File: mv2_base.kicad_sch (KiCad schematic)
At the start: 60 parts, among them J1 Conn_01x20, J2 OLED, U1 TPS65130RGE

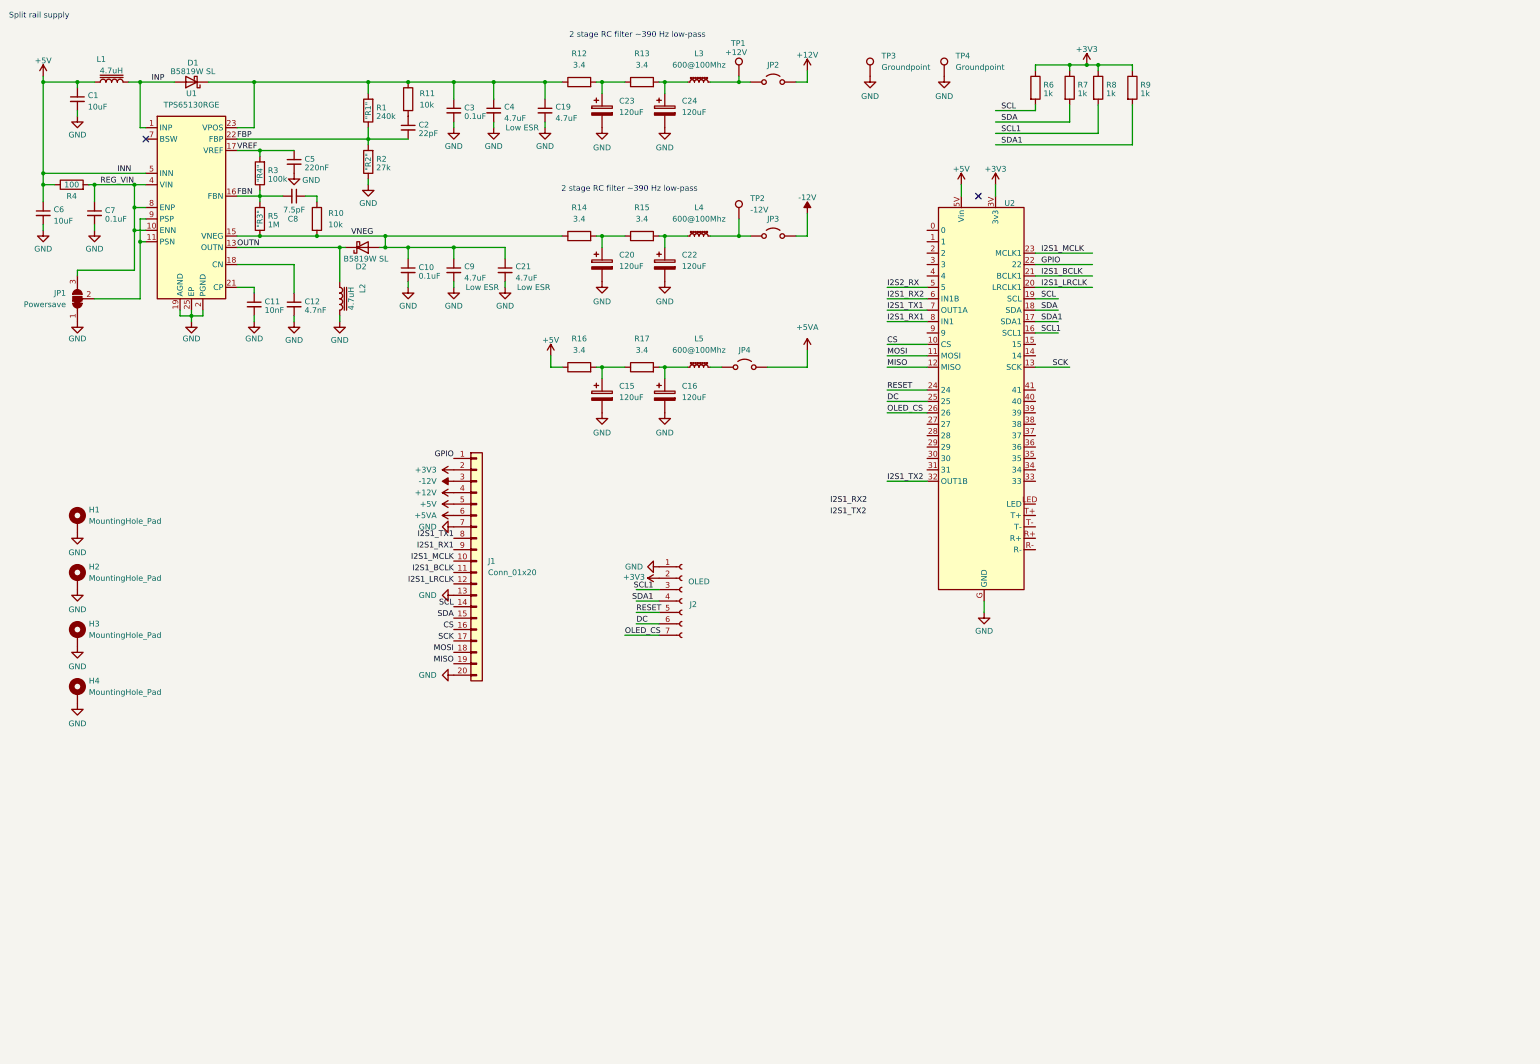
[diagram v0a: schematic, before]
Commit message: New filters
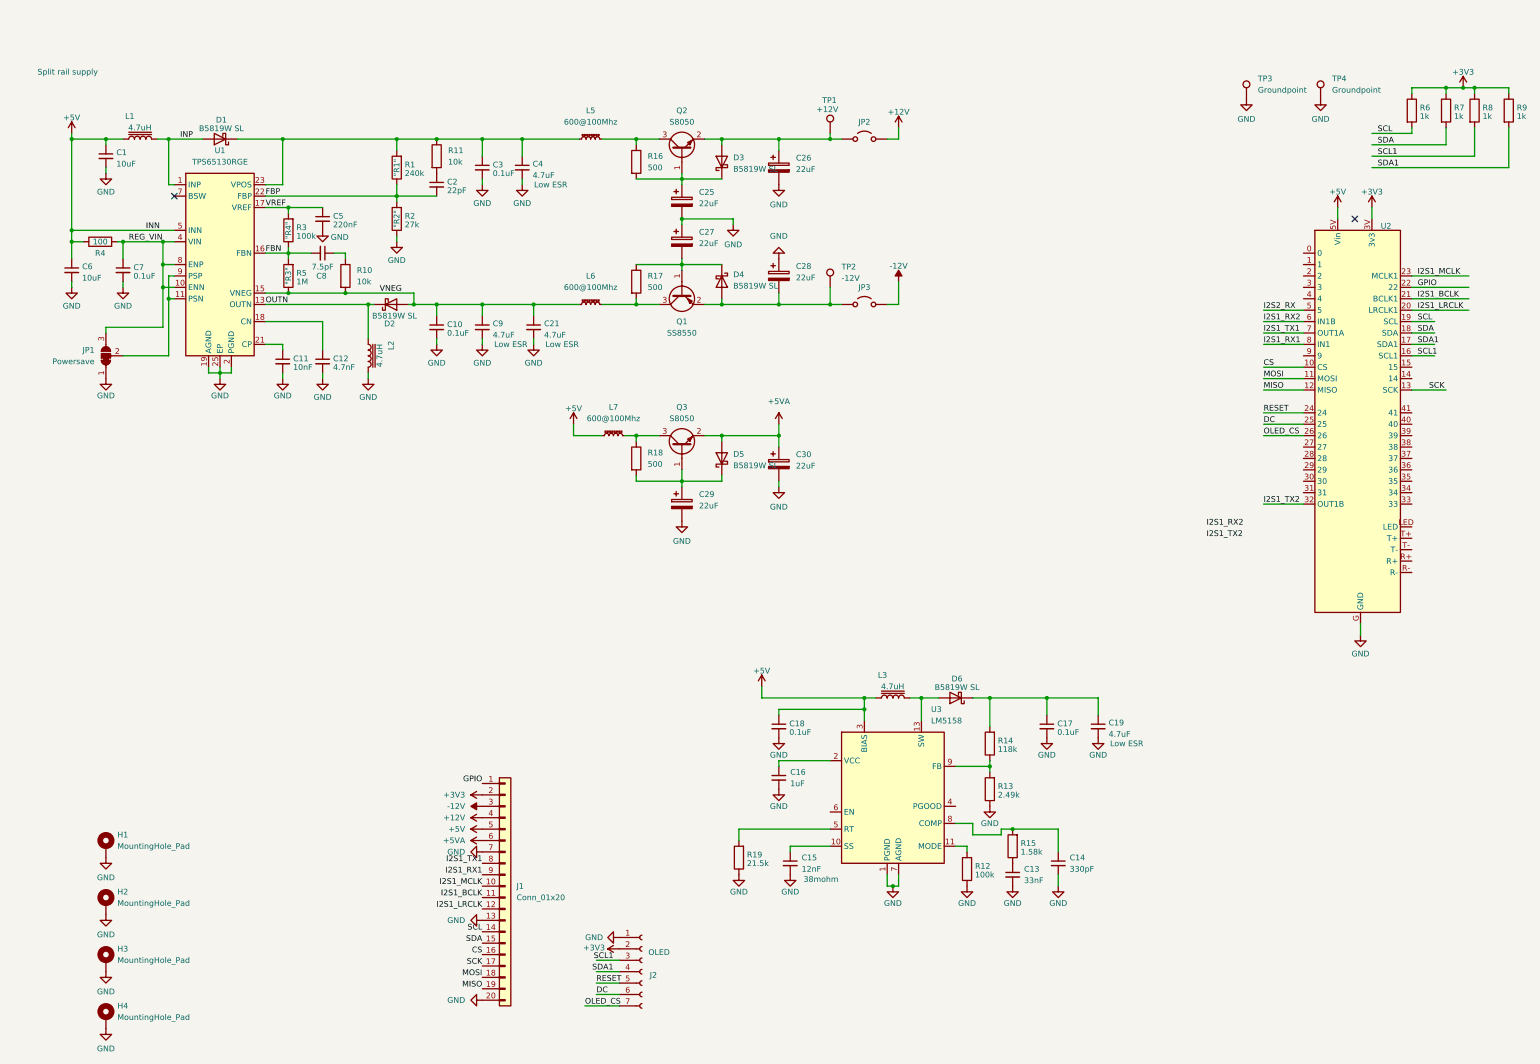
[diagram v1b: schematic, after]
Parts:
- removed C15, C16, C20, C22, C23, C24: 120uF, Capacitor_SMD:CP_Elec_6.3x7.7, symbol Device:C_Polarized
- removed JP4: Jumper_2_Open, Connector_PinHeader_2.54mm:PinHeader_1x02_P2.54mm_Vertical, symbol Jumper:Jumper_2_Open
- removed L3, L4: 600@100Mhz, Inductor_SMD:L_0603_1608Metric, symbol Device:L_Ferrite_Small
- added C13: 33nF, Capacitor_SMD:C_0603_1608Metric_Pad1.08x0.95mm_HandSolder, symbol Device:C_Small
- added C14: 330pF, Capacitor_SMD:C_0603_1608Metric_Pad1.08x0.95mm_HandSolder, symbol Device:C_Small
- added C15: 12nF, Capacitor_SMD:C_0603_1608Metric_Pad1.08x0.95mm_HandSolder, symbol Device:C_Small
- added C16: 1uF, Capacitor_SMD:C_0805_2012Metric_Pad1.18x1.45mm_HandSolder, symbol Device:C_Small
- added C17, C18: 0.1uF, Capacitor_SMD:C_0402_1005Metric, symbol Device:C_Small
- added C25, C26, C27, C28, C29, C30: 22uF, Capacitor_SMD:C_0805_2012Metric, symbol Device:C_Polarized
- added D3, D4, D5, D6: B5819W SL, Diode_SMD:D_SOD-123, symbol Device:D_Schottky
- added L3: 4.7uH, Inductor_SMD:L_Wuerth_WE-TPC-3816, symbol Device:L_Iron
- added L6, L7: 600@100Mhz, Inductor_SMD:L_0603_1608Metric, symbol Device:L_Ferrite_Small
- added Q1: SS8550, Package_TO_SOT_SMD:SOT-23, symbol Transistor_BJT:Q_PNP_BEC
- added Q2, Q3: S8050, Package_TO_SOT_SMD:SOT-23, symbol Transistor_BJT:Q_NPN_BEC
- added R18: 500, Resistor_SMD:R_0402_1005Metric, symbol Device:R
- added R19: 21.5k, Resistor_SMD:R_0402_1005Metric, symbol Device:R
- added U3: LM5158, symbol Library:LM5158
- C19: footprint Capacitor_SMD:C_0805_2012Metric_Pad1.18x1.45mm_HandSolder -> Capacitor_SMD:C_0805_2012Metric; DatasheetRef C4 -> C5
- R12: value 3.4 -> 100k; footprint Resistor_SMD:R_0603_1608Metric -> Resistor_SMD:R_0402_1005Metric; LCSC C22939 -> C25803; Part R 3.4Ω 125mW 1% 0603 -> (none); Shop https://eu.mouser.com/ProductDetail/YAGEO/RC0603FR-073R4L?q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 -> (none)
- R13: value 3.4 -> 2.49k; footprint Resistor_SMD:R_0603_1608Metric -> Resistor_SMD:R_0402_1005Metric; LCSC C22939 -> C25803; Part R 3.4Ω 125mW 1% 0603 -> (none); Shop https://eu.mouser.com/ProductDetail/YAGEO/RC0603FR-073R4L?q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 -> (none)
- R14: value 3.4 -> 118k; footprint Resistor_SMD:R_0603_1608Metric -> Resistor_SMD:R_0402_1005Metric; LCSC C22939 -> C25803; Part R 3.4Ω 125mW 1% 0603 -> (none); Shop https://eu.mouser.com/ProductDetail/YAGEO/RC0603FR-073R4L?q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 -> (none)
- R15: value 3.4 -> 1.58k; footprint Resistor_SMD:R_0603_1608Metric -> Resistor_SMD:R_0402_1005Metric; LCSC C22939 -> C25803; Part R 3.4Ω 125mW 1% 0603 -> (none); Shop https://eu.mouser.com/ProductDetail/YAGEO/RC0603FR-073R4L?q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 -> (none)
- R16, R17: value 3.4 -> 500; footprint Resistor_SMD:R_0603_1608Metric -> Resistor_SMD:R_0402_1005Metric; LCSC C22939 -> (none); Part R 3.4Ω 125mW 1% 0603 -> (none); Shop https://eu.mouser.com/ProductDetail/YAGEO/RC0603FR-073R4L?q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 -> (none)
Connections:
- net +5V: now also C18.1, L3.2, L7.1, U3.3 (BIAS); no longer R16.1
- net +5VA: now also C30.1, D5.2 (A), Q3.2 (E)
- net GND: now also R12.1, R13.1, C13.2, C14.2, C15.2, C16.2, C17.2, C18.2, C25.2, C26.2, C27.1, C28.1, C29.2, C30.2, R19.1, U3.1 (PGND), U3.16 (PGND), U3.7 (AGND)
- net VNEG: now also L6.1; no longer R14.1
- net at R15.1: now also C13.1; no longer R14.2
- net at JP2.1 (A), TP1.1: now also C26.1, D3.2 (A), Q2.2 (E)
- net at R16.2: now also C25.1, D3.1 (K), Q2.1 (B); no longer R17.1
- net at L5.2: now also R16.1, Q2.3 (C)
- net at R13.2: now also R14.1, U3.9 (FB)
- net at JP3.1 (A), TP2.1: now also C28.2, D4.2 (A), Q1.2 (E)
- net at R17.2: now also L6.2, Q1.3 (C); no longer L5.1
- net at C3.1, C4.1, D1.1 (K)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: now also L5.1; no longer C19.1, R12.1
- net at R12.2: now also U3.11 (MODE); no longer R13.1
- net at R15.2: now also C14.1, U3.8 (COMP)
- new net: L7.2, Q3.3 (C), R18.1
- new net: C15.1, U3.10 (SS)
- new net: D6.2 (A), L3.1, U3.13 (SW), U3.14 (SW)
- new net: C16.1, U3.2 (VCC)
- new net: R19.2, U3.5 (RT)
- new net: C17.1, C19.1, D6.1 (K), R14.2
- new net: C29.1, D5.1 (K), Q3.1 (B), R18.2
- new net: C27.2, D4.1 (K), Q1.1 (B), R17.1
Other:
- note removed: "2 stage RC filter ~390 Hz low-pass"
- moved on the sheet: C1, C10, C11, C12, C2, C21, C3, C4, C5, C6, C7, C8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
